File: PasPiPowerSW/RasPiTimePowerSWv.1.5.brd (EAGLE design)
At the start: 100 x 80 mm, 38 parts, among them IC1 MSP430G2553, IC2 NJM2845DL1-33, J1 3P Socket, J2 3P Socket, Q1 P-ch MOS FET, T1 2SC1815-Y

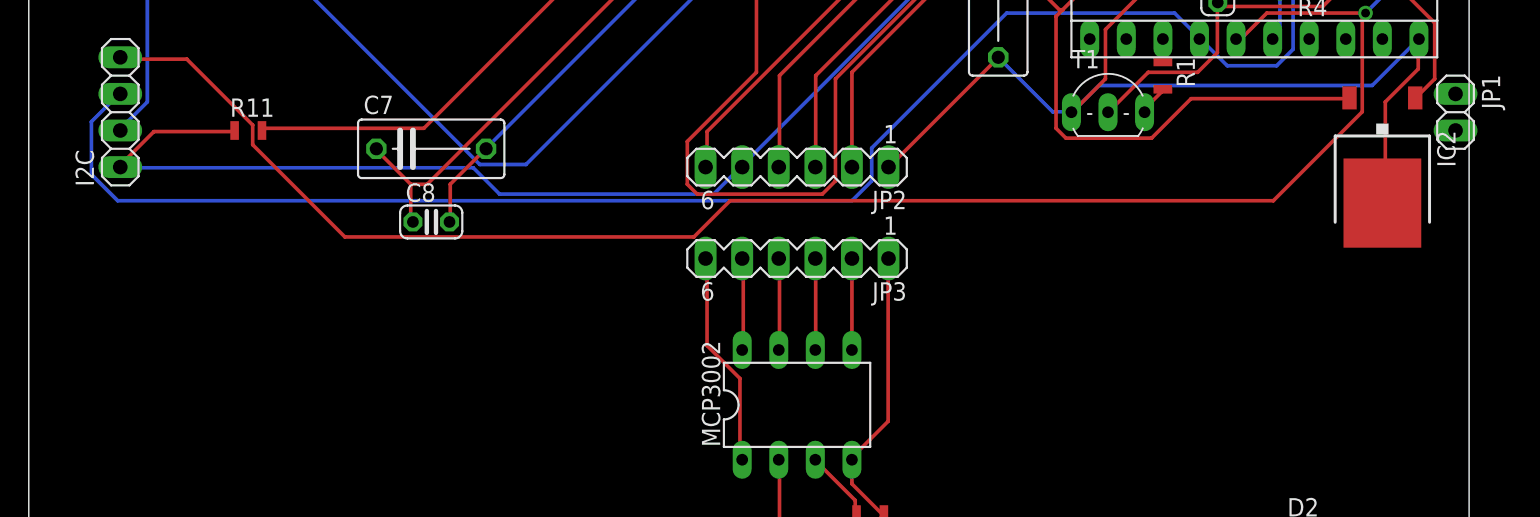
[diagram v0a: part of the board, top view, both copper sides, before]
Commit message: Replaced TO-252 Voltage Regulator part
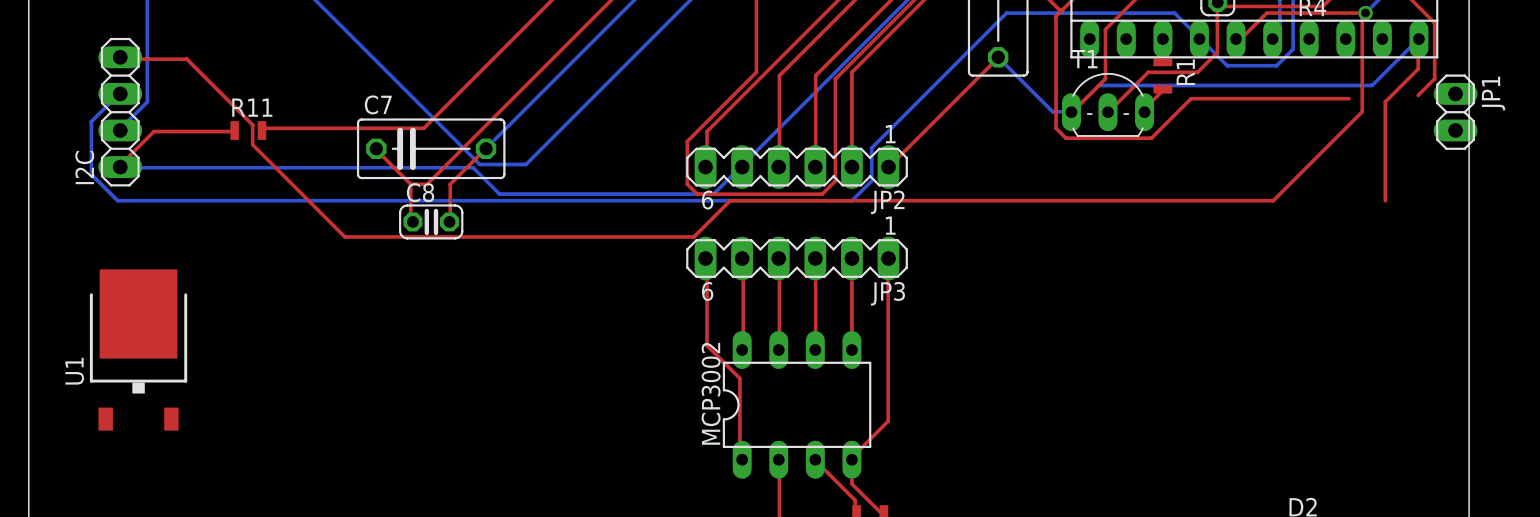
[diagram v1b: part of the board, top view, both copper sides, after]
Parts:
- removed IC2: NJM2845DL1-33, linear:TO252
- added U1: +12v, SparkFun-IC-Power:TO-252
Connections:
- net 3.3V: now also U1.2; no longer IC2.2
- net 5VIN: now also U1.1; no longer IC2.1
- net GND: now also U1.3; no longer IC2.3

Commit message: Revert "revert to NJM2845DL1"
This reverts commit ec86f7a8aa55efb6e9586fa3a205028523492dc4.
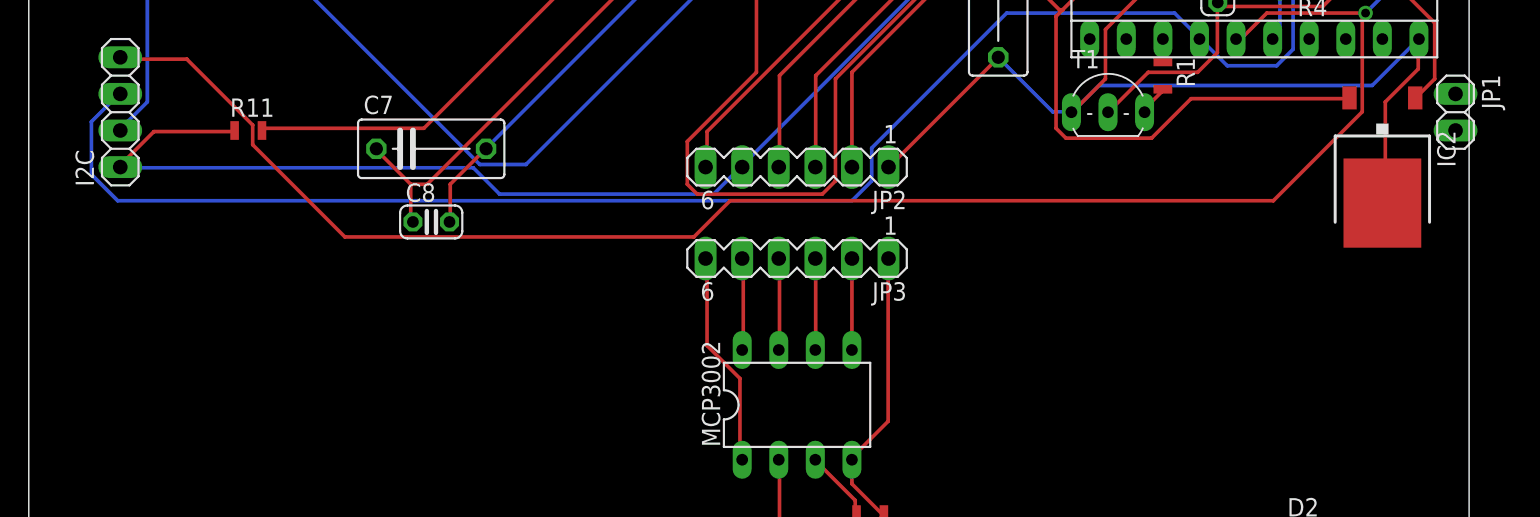
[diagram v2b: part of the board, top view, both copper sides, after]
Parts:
- removed U1: +12v, SparkFun-IC-Power:TO-252
- added IC2: NJM2845DL1-33, linear:TO252
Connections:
- net 3.3V: now also IC2.2; no longer U1.2
- net 5VIN: now also IC2.1; no longer U1.1
- net GND: now also IC2.3; no longer U1.3
